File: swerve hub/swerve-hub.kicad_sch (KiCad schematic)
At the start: 4 parts

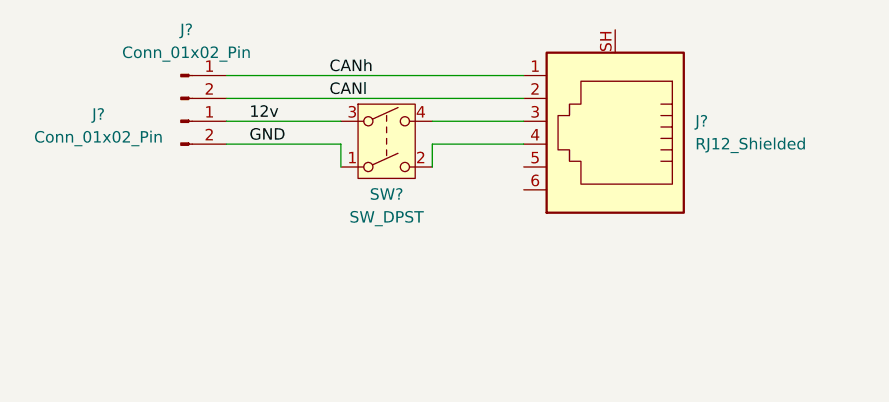
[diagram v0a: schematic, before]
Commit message: canivore hub mostly done
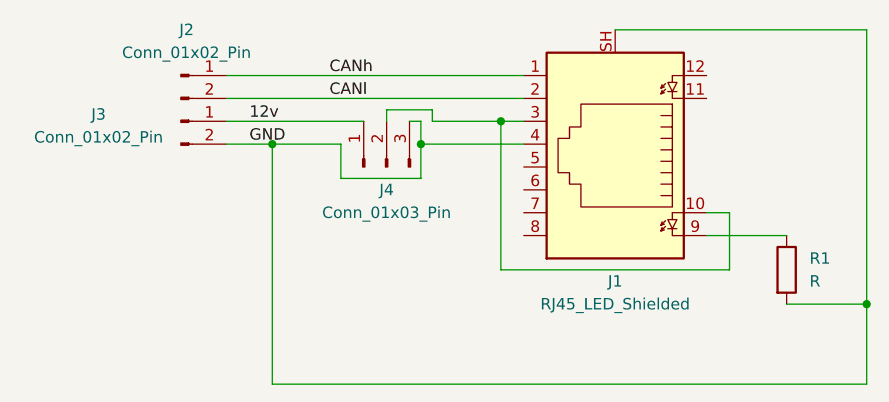
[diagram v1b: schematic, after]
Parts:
- removed J?: RJ12_Shielded, symbol Connector:RJ12_Shielded
- removed SW?: SW_DPST, symbol Switch:SW_DPST
- added J1: RJ45_LED_Shielded, MTJ_88ARX1_FSM_LG:ADAMTECH_MTJ-88ARX1-FSM-LG, symbol Connector:RJ45_LED_Shielded
- added J4: Conn_01x03_Pin, Connector_PinHeader_2.54mm:PinHeader_1x03_P2.54mm_Horizontal, symbol Connector:Conn_01x03_Pin
- added R1: R, Resistor_THT:R_Axial_DIN0207_L6.3mm_D2.5mm_P10.16mm_Horizontal, symbol Device:R
- J2, J3: renamed from J?; footprint (none) -> TerminalBlock_WAGO:TerminalBlock_WAGO_2601-1102_1x02_P3.50mm_Horizontal
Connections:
- net 12v: now also J4.1 (Pin_1)
- net CANh: now also J1.1
- net CANl: now also J1.2
- net GND: now also J1.4, J1.SH, J4.3 (Pin_3), R1.2
- new net: J1.10, J1.3, J4.2 (Pin_2)
- new net: J1.9, R1.1
